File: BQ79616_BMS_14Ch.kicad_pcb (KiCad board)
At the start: 2 copper layers, 100 x 60 mm, 155 parts, among them J1 Conn_02x10_Odd_Even, J2 Conn_02x10_Odd_Even, J3 Conn_Therm, J4 BMS_A_IN, J5 BMS_A_OUT, Q1 MMBT5551

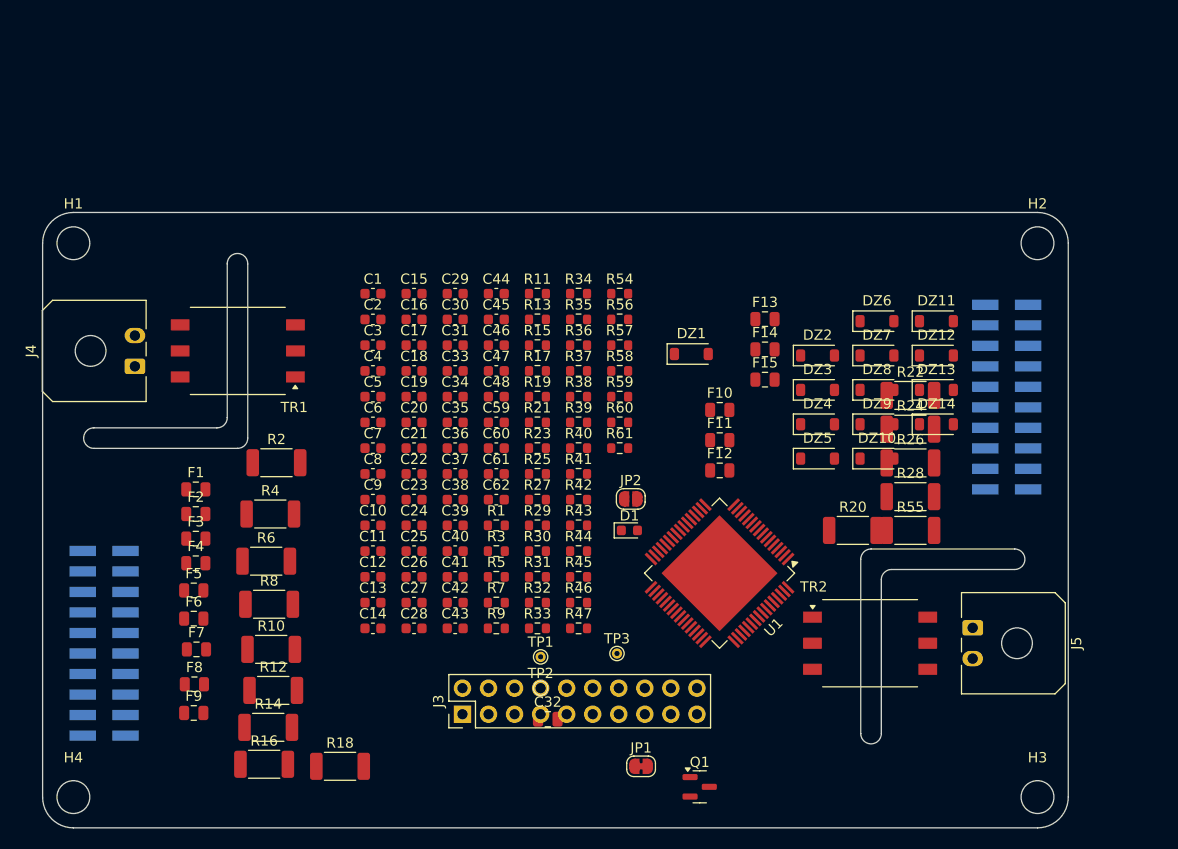
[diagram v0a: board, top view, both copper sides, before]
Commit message: Finish positioning of all components Ver1ST
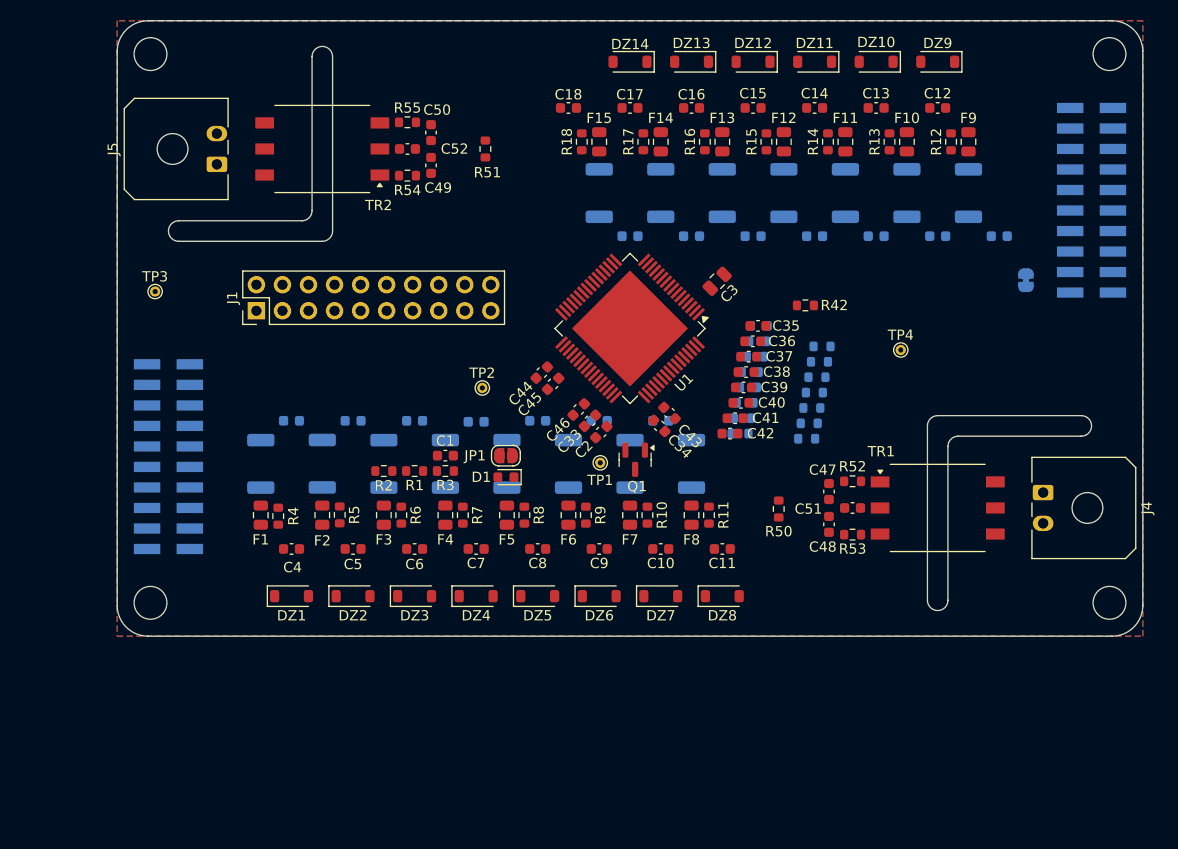
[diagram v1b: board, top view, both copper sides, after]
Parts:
- added TP1: TestPoint, TestPoint:TestPoint_THTPad_D1.0mm_Drill0.5mm, F.Cu at (147.1, 103.1)
- C19: renamed from C29; moved to B.Cu
- C20: renamed from C28; moved to B.Cu
- C21: renamed from C27; moved to B.Cu
- C22: renamed from C26; moved to B.Cu
- C23: renamed from C25; moved to B.Cu
- C24: moved to B.Cu
- C25: renamed from C23; moved to B.Cu
- C26: renamed from C22; moved to B.Cu
- C27: renamed from C21; moved to B.Cu
- C28: renamed from C20; moved to B.Cu
- C29: renamed from C19; moved to B.Cu
- C30: renamed from C18; moved to B.Cu
- C31: renamed from C17; moved to B.Cu
- C32: renamed from C16; moved to B.Cu
- JP2: renamed from JP1; moved to B.Cu
- R19: renamed from R2; moved to B.Cu
- R20: renamed from R4; moved to B.Cu
- R21: renamed from R6; moved to B.Cu
- R22: renamed from R8; moved to B.Cu
- R23: renamed from R10; moved to B.Cu
- R24: renamed from R12; moved to B.Cu
- R25: renamed from R14; moved to B.Cu
- R26: renamed from R16; moved to B.Cu
- R27: renamed from R18; moved to B.Cu
- R28: renamed from R20; moved to B.Cu
- R29: renamed from R22; moved to B.Cu
- R30: renamed from R24; moved to B.Cu
- R31: renamed from R26; moved to B.Cu
- R32: renamed from R28; moved to B.Cu
- R33: renamed from R55; moved to B.Cu
- R34: renamed from R32; moved to B.Cu
- R35: renamed from R33; moved to B.Cu
- R36: renamed from R34; moved to B.Cu
- R37: renamed from R35; moved to B.Cu
- R38: renamed from R36; moved to B.Cu
- R39: renamed from R37; moved to B.Cu
- R40: renamed from R38; moved to B.Cu
- R41: renamed from R39; moved to B.Cu
- R43: renamed from R41; moved to B.Cu
- R44: renamed from R42; moved to B.Cu
- R45: renamed from R43; moved to B.Cu
- R46: renamed from R44; moved to B.Cu
- R47: renamed from R45; moved to B.Cu
- R48: renamed from R46; moved to B.Cu
- R49: renamed from R47; moved to B.Cu
- moved H1 102.7 mm to (196.8, 63.2)
- moved F9 93.8 mm to (183.0, 71.8), turned to -90 degrees
- moved H2 88.4 mm to (103.2, 63.2)
- moved R27 82.9 mm to (183.0, 76.8), turned to -90 degrees
- moved DZ1 65.1 mm to (117.0, 116.1)
- moved C12 64.3 mm to (180.0, 68.5), turned to 180 degrees
- moved C26 61.6 mm to (186.0, 81.0), turned to 180 degrees
- moved JP2 60.4 mm to (188.6, 85.3), turned to 90 degrees
- moved DZ2 60.3 mm to (123.0, 116.1)
- moved C13 57.9 mm to (174.0, 68.5), turned to 180 degrees
- moved DZ3 56.0 mm to (129.0, 116.1)
- moved C27 55.1 mm to (180.0, 81.0), turned to 180 degrees
- moved TP3 53.9 mm to (103.7, 86.4)
- moved DZ4 52.3 mm to (135.0, 116.1)
- moved C14 51.4 mm to (168.0, 68.5), turned to 180 degrees
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- renumbered C33 to C1, C9 to C10, C8 to C11, C7 to C12, C6 to C13, C5 to C14, C4 to C15, C3 to C16, C2 to C17, C1 to C18, C34 to C2, C32 to C3, C35 to C33, C36 to C34, C41 to C35, C42 to C36, C43 to C37, C44 to C38, C45 to C39, C15 to C4, C46 to C40, C47 to C41, C48 to C42, C40 to C43, C37 to C44, C38 to C45, C39 to C46, C31 to C47, C61 to C48, C59 to C49, C14 to C5, C60 to C50, C62 to C51, C30 to C52, C13 to C6, C12 to C7, C11 to C8, C10 to C9, DZ14 to DZ1, DZ5 to DZ10, DZ4 to DZ11, DZ3 to DZ12, DZ2 to DZ13, DZ1 to DZ14, DZ13 to DZ2, DZ12 to DZ3, DZ11 to DZ4, DZ10 to DZ5, DZ9 to DZ6, DZ8 to DZ7, DZ7 to DZ8, DZ6 to DZ9, J3 to J1, J1 to J2, J2 to J3, J5 to J4, J4 to J5, JP2 to JP1, R31 to R1, R13 to R10, R15 to R11, R17 to R12, R19 to R13, R21 to R14, R23 to R15, R25 to R16, R27 to R17, R54 to R18, R29 to R2, R30 to R3, R1 to R4, R40 to R42, R3 to R5, R59 to R50, R58 to R51, R60 to R52, R61 to R53, R56 to R54, R57 to R55, R5 to R6, R9 to R8, R11 to R9, TP1 to TP2, TP2 to TP3, TP3 to TP4, TR2 to TR1, TR1 to TR2
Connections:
- C45 pad 1: /ADVV_A -> /AVDD_A
- J2 pad 17: /CELL_A6 -> unconnected-(J2-Pin_17-Pad17)
- J3 pad 1: /CELL_A5 -> /CELL_A6
- J3 pad 12: GND1 -> /CELL_A1
- J3 pad 13: /RX_A -> GND1
- J3 pad 16: /TX_A -> /RX_A
- J3 pad 17: /CVDD_A -> /TX_A
- J3 pad 20: unconnected-(J2-Pin_20-Pad20) (its old number) -> /CVDD_A
- J3 pad 4: /CELL_A4 -> /CELL_A5
- J3 pad 5: /CELL_A3 -> /CELL_A4
- J3 pad 8: /CELL_A2 -> /CELL_A3
- J3 pad 9: /CELL_A1 -> /CELL_A2
- U1 pad 38: /ADVV_A -> /AVDD_A
- U1 pad 49: /ADVV_A -> /DVDD_A
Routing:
- added copper zone on B.Cu, net GND1
- added copper zone on F.Cu, net GND1
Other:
- outline, holes or cut-outs redrawn
